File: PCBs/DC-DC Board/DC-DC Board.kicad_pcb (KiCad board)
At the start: 2 copper layers, 58.4 x 36.8 mm, 38 parts, among them J1 Conn_01x01, J2 Conn_01x01, J3 Conn_01x01, J4 Conn_01x01, J5 Conn_01x02, J6 Conn_01x02, Q1 Q_NMOS_GDS, U1 DBQ0135V2, U2 ACS711, U3 NCP551, U4 TLV733P

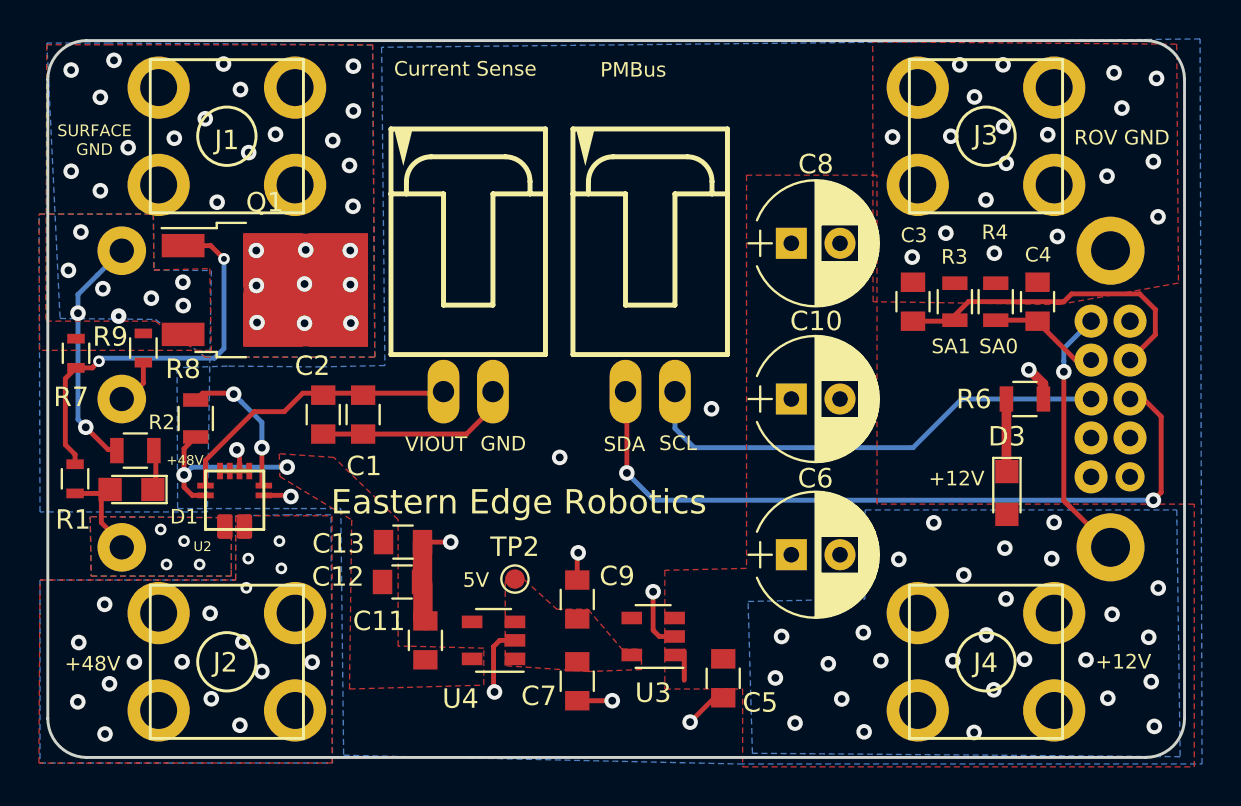
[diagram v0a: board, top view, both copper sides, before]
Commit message: DC-DC Mirco Updates
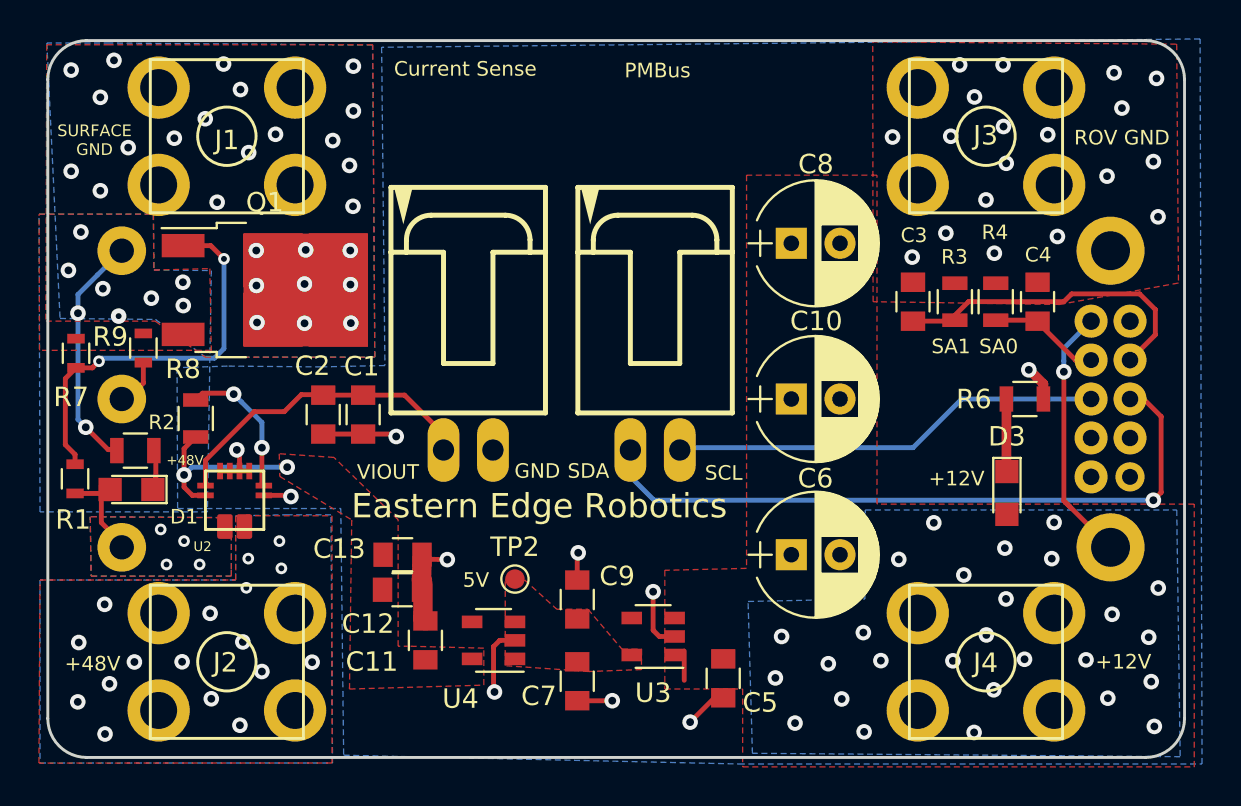
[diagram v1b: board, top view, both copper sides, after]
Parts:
- moved J5 3.01 mm to (102.0, 45.0)
- moved J6 3.00 mm to (92.4, 45.0)
- moved C13 0.65 mm to (89.0, 58.0)
- moved C12 0.40 mm to (89.0, 59.8)
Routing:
- net GND: track 35.1 -> 27.0 mm, vias 30 -> 29
- net SDA: track 38.3 -> 34.1 mm, vias 2 -> 1
- net SCL: track 24.7 -> 21.4 mm
- net VIOUT: track 15.0 -> 16.6 mm
